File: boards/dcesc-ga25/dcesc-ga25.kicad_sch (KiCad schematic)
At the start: 11 parts, among them J1 Conn_01x03, J2 Conn_01x03, U1 CH32V003J4M6

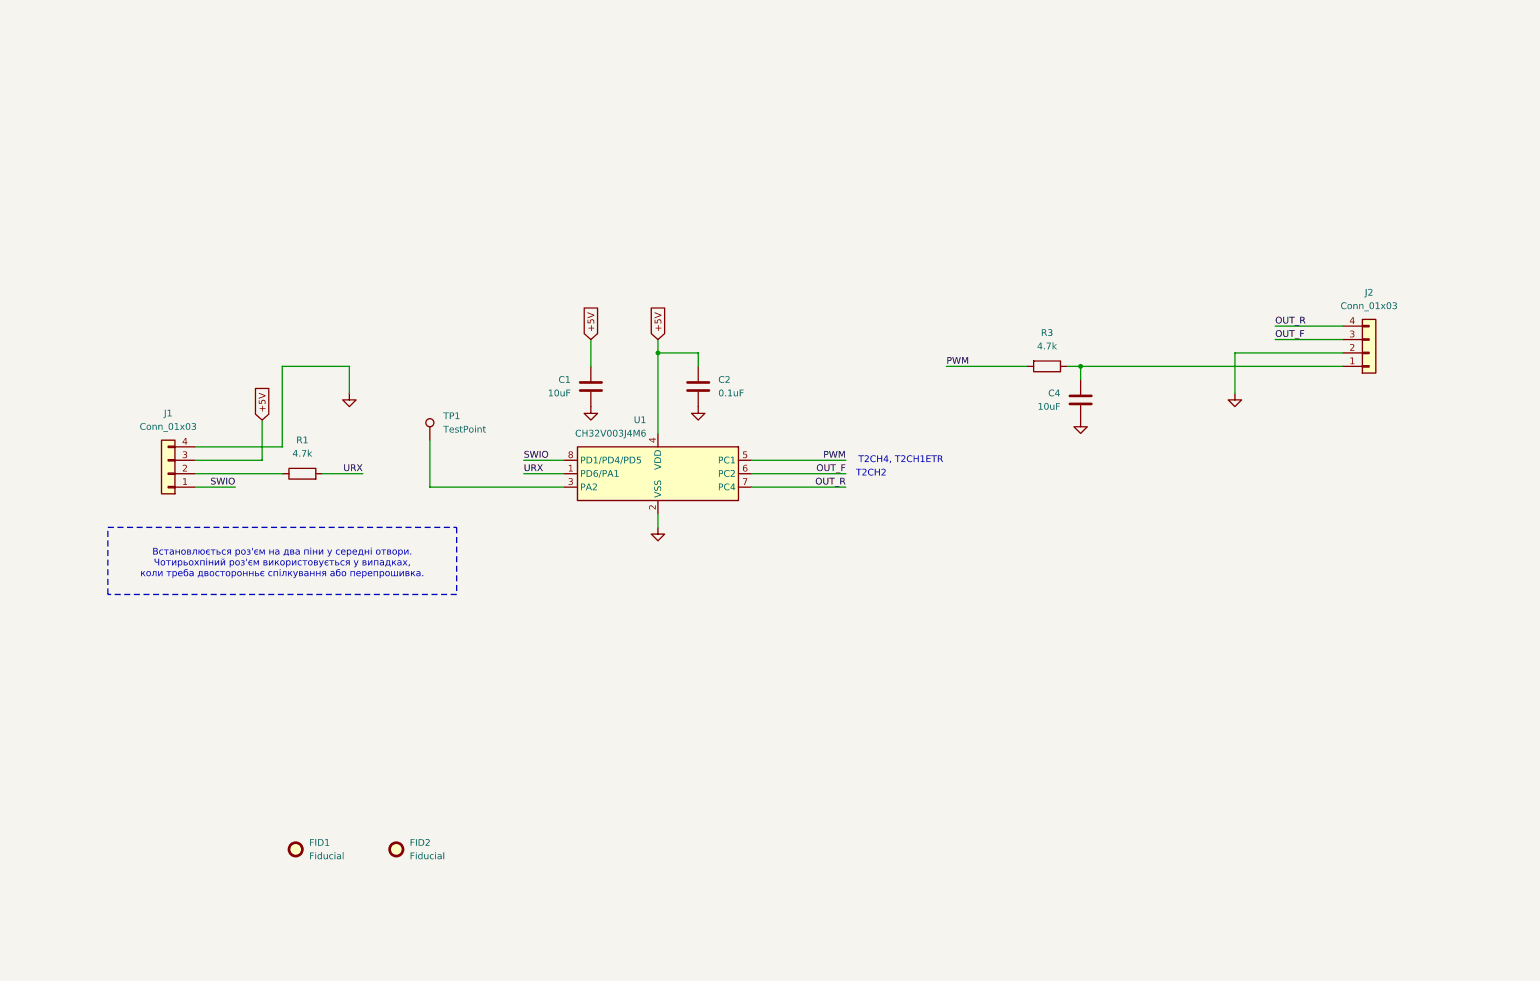
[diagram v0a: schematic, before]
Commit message: Розведено.
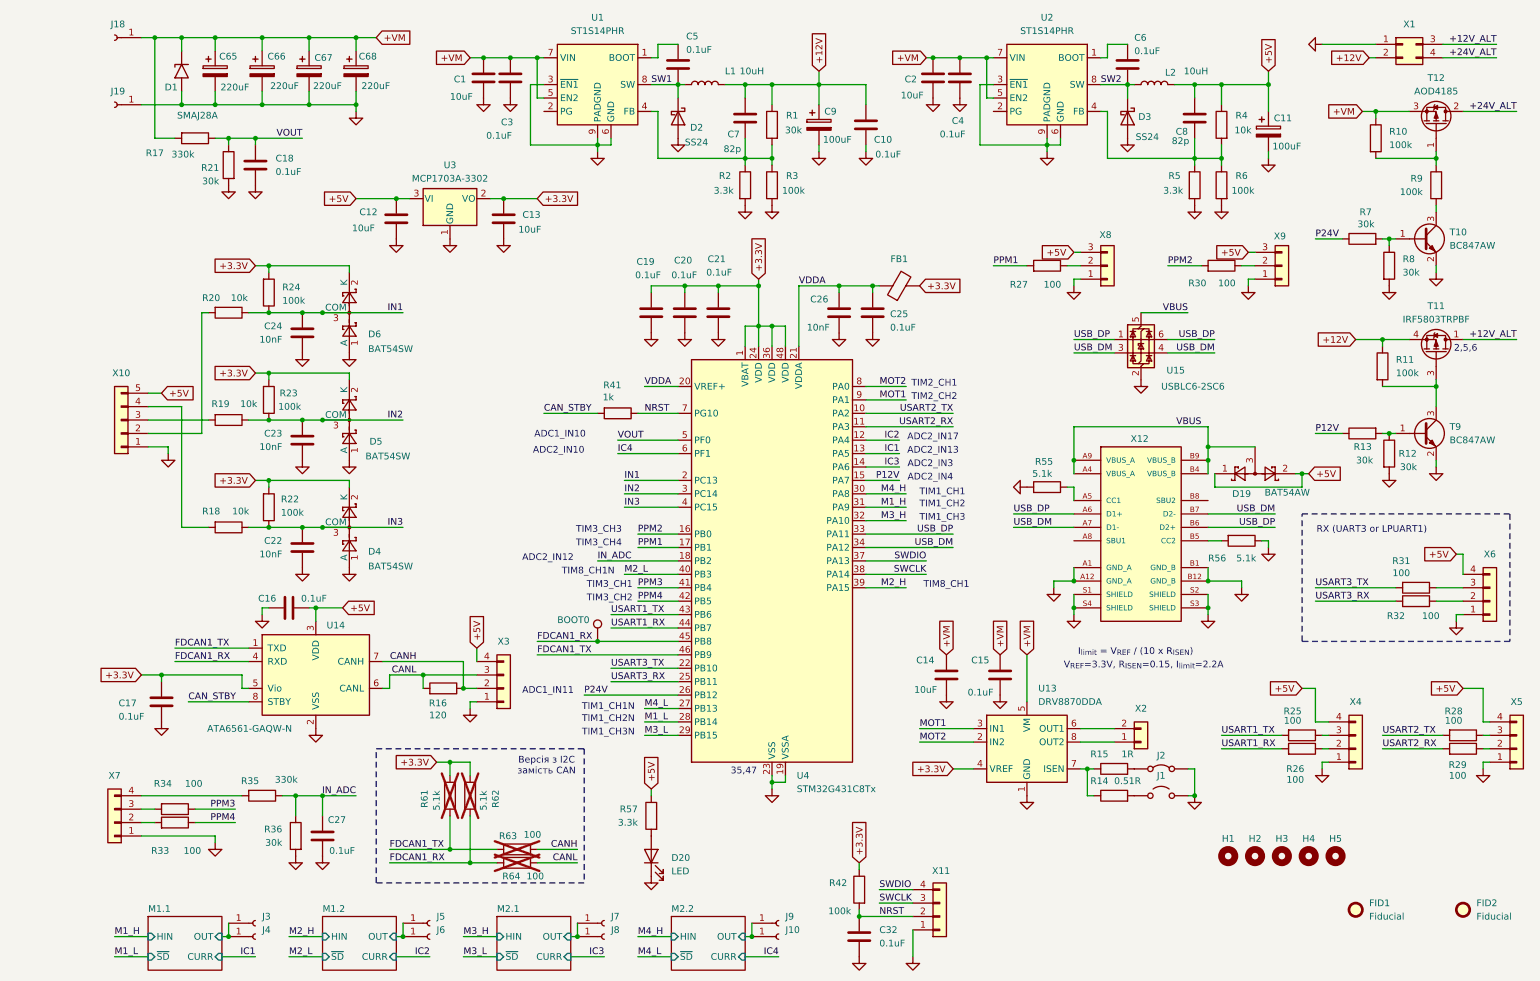
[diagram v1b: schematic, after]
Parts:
- removed J2: Conn_01x03, Connector_JST:JST_PH_S4B-PH-K_1x04_P2.00mm_Horizontal, symbol Connector_Generic:Conn_01x04
- removed U1: CH32V003J4M6, Package_SO:SOP-8_3.9x4.9mm_P1.27mm, symbol MCU_WCH_CH32V0:CH32V003JxMx
- added C1, C14: 10uF, Capacitor_SMD:C_1206_3216Metric, symbol Device:C
- added C10, C15, C16, C17, C18, C19, C20, C21, C25, C27, C3, C32, C5, C6: 0.1uF, Capacitor_SMD:C_0603_1608Metric, symbol Device:C
- added C11: 100uF, Capacitor_Tantalum_SMD:CP_EIA-3528-12_Kemet-T, symbol Device:C_Polarized
- added C12, C13: 10uF, Capacitor_SMD:C_0805_2012Metric, symbol Device:C
- added C22, C23, C24: 10nF, Capacitor_SMD:C_0603_1608Metric, symbol Device:C
- added C65, C66, C67, C68: 220uF, Capacitor_THT:CP_Radial_D10.0mm_P5.00mm, symbol Device:C_Polarized
- added C7, C8: 82p, Capacitor_SMD:C_0603_1608Metric, symbol Device:C
- added C9: 100uF, Capacitor_Tantalum_SMD:CP_EIA-7343-15_Kemet-W, symbol Device:C_Polarized
- added D1: SMAJ28A, Diode_SMD:D_SMA, symbol Diode:SMAJ28A
- added D19: BAT54AW, Package_TO_SOT_SMD:SOT-323_SC-70, symbol Diode:BAT54AW
- added D2, D3: SS24, Diode_SMD:D_SMA, symbol Diode:SS24
- added D20: LED, LED_SMD:LED_0805_2012Metric, symbol Device:LED
- added D4, D5, D6: BAT54SW, Package_TO_SOT_SMD:SOT-323_SC-70, symbol Diode:BAT54SW
- added FB1: FerriteBead, Inductor_SMD:L_0603_1608Metric, symbol Device:FerriteBead
- added H1, H2, H3, H4, H5: MountingHole, MountingHole:MountingHole_3.2mm_M3, symbol Mechanical:MountingHole
- added J1: Jumper_2_Open, Jumper:SolderJumper-2_P1.3mm_Open_RoundedPad1.0x1.5mm, symbol Jumper:Jumper_2_Open
- added J10, J3, J4, J5, J6, J7, J8, J9: Conn_01x01_Socket, Connector_Wire:SolderWire-2.5sqmm_1x01_D2.4mm_OD4.4mm, symbol Connector:Conn_01x01_Socket
- added J18, J19: Conn_01x01_Socket, Connector_Wire:SolderWire-6sqmm_1x01_D3.5mm_OD7mm, symbol Connector:Conn_01x01_Socket
- added J2: Jumper_2_Bridged, Jumper:SolderJumper-2_P1.3mm_Bridged_RoundedPad1.0x1.5mm, symbol Jumper:Jumper_2_Bridged
- added L1, L2: 10uH, locals:Inductor_NR6028T100M, symbol Device:L
- added R10, R11, R22, R23, R24, R42, R6, R9: 100k, Resistor_SMD:R_0603_1608Metric, symbol Device:R
- added R12, R13, R21, R36, R7, R8: 30k, Resistor_SMD:R_0603_1608Metric, symbol Device:R
- added R14: 0.51R, Resistor_SMD:R_1206_3216Metric, symbol Device:R
- added R15: 1R, Resistor_SMD:R_1206_3216Metric, symbol Device:R
- added R16: 120, Resistor_SMD:R_0603_1608Metric, symbol Device:R
- added R17, R35: 330k, Resistor_SMD:R_0603_1608Metric, symbol Device:R
- added R18, R19, R20, R4: 10k, Resistor_SMD:R_0603_1608Metric, symbol Device:R
- added R2, R5, R57: 3.3k, Resistor_SMD:R_0603_1608Metric, symbol Device:R
- added R25, R26, R27, R28, R29, R30, R31, R32, R33, R34, R63, R64: 100, Resistor_SMD:R_0603_1608Metric, symbol Device:R
- added R41: 1k, Resistor_SMD:R_0603_1608Metric, symbol Device:R
- added R55, R56, R61, R62: 5.1k, Resistor_SMD:R_0603_1608Metric, symbol Device:R
- added T10, T9: BC847AW, Package_TO_SOT_SMD:SOT-323_SC-70, symbol Transistor_BJT:BC847W
- added T11: IRF5803TRPBF, Package_SO:TSOP-6_1.65x3.05mm_P0.95mm, symbol Transistor_FET:IRFTS9342PBF
- added T12: AOD4185, Package_TO_SOT_SMD:TO-252-2, symbol Transistor_FET:SUD45P03-09
- added U1, U2: ST1S14PHR, Package_SO:TI_SO-PowerPAD-8, symbol Regulator_Switching:ST1S14PHR
- added U13: DRV8870DDA, Package_SO:Texas_HTSOP-8-1EP_3.9x4.9mm_P1.27mm_EP2.95x4.9mm_Mask2.4x3.1mm_ThermalVias, symbol Driver_Motor:DRV8870DDA
- added U14: ATA6561-GAQW-N, Package_SO:SOIC-8_3.9x4.9mm_P1.27mm, symbol Interface_CAN_LIN:MCP2562-E-SN
- added U15: USBLC6-2SC6, Package_TO_SOT_SMD:SOT-23-6, symbol Power_Protection:USBLC6-2SC6
- added U3: MCP1703A-3302, locals:MCP1703, symbol LocalBaden:MCP1703A-3302_SOT23-regul_0
- added U4: STM32G431C8Tx, Package_QFP:LQFP-48_7x7mm_P0.5mm, symbol MCU_ST_STM32G4:STM32G431C8Tx
- added X1: Conn_02x02_Top_Bottom, Connector_Molex:Molex_Micro-Fit_3.0_43045-0412_2x02_P3.00mm_Vertical, symbol Connector_Generic:Conn_02x02_Top_Bottom
- added X11, X3, X4, X5, X6, X7: Conn_01x03, Connector_JST:JST_ZH_B4B-ZR_1x04_P1.50mm_Vertical, symbol Connector_Generic:Conn_01x04
- added X12: USB4120-03-C_REVA, locals:GCT_USB4120-03-C_REVA, symbol USB4120-03-C_REVA:USB4120-03-C_REVA
- added X2: Conn_01x03, Connector_JST:JST_XH_B2B-XH-AM_1x02_P2.50mm_Vertical, symbol Connector_Generic:Conn_01x02
- added X8, X9: Conn_01x03, Connector_JST:JST_ZH_B3B-ZR_1x03_P1.50mm_Vertical, symbol Connector_Generic:Conn_01x03
- C2: value 0.1uF -> 10uF; footprint Capacitor_SMD:C_0603_1608Metric -> Capacitor_SMD:C_1206_3216Metric
- C26: renamed from C1; value 10uF -> 10nF; footprint Capacitor_SMD:C_0805_2012Metric -> Capacitor_SMD:C_0603_1608Metric
- C4: value 10uF -> 0.1uF; footprint Capacitor_SMD:C_0805_2012Metric -> Capacitor_SMD:C_0603_1608Metric
- R1: value 4.7k -> 30k
- R3: value 4.7k -> 100k
- TP1: value TestPoint -> BOOT0; footprint TestPoint:TestPoint_Pad_2.0x2.0mm -> TestPoint:TestPoint_Pad_1.0x1.0mm
- X10: renamed from J1; footprint Connector_JST:JST_PH_S4B-PH-K_1x04_P2.00mm_Horizontal -> Connector_JST:JST_ZH_B5B-ZR_1x05_P1.50mm_Vertical; symbol Connector_Generic:Conn_01x04 -> Connector_Generic:Conn_01x05
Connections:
- net PWM is gone; now on net GND: R3.2
- net SWIO is gone; now on net GND: X10.1 (Pin_1)
- net URX is gone; now on an unnamed net: R1.2
- net +5V: now also X10.5 (Pin_5), C11.1, C12.1, C16.1, C8.1, D19.1, D19.2, L2.2, R4.1, R57.1, U14.3 (VDD), U3.3 (VI), X3.4 (Pin_4), X4.4 (Pin_4), X5.4 (Pin_4), X6.4 (Pin_4), X8.3 (Pin_3), X9.3 (Pin_3); no longer C2.1, C26.1, X10.3 (Pin_3)
- net GND: now also C1.2, C10.2, C11.2, C12.2, C13.2, C14.2, C15.2, C16.2, C17.2, C18.2, C19.2, C20.2, C21.2, C22.2, C23.2, C24.2, C25.2, C27.2, C3.2, C32.2, C65.2, C66.2, C67.2, C68.2, C9.2, D1.2 (A2), D2.2 (A), D20.1 (K), D3.2 (A), D4.1 (A), D5.1 (A), D6.1 (A), J1.2 (B), J19.1 (Pin_1), J2.2 (B), R12.2, R2.2, R21.2, R36.2, R5.2, R55.2, R56.1, R6.2, R8.2, T10.2 (E), T9.2 (E), U1.3 (~{EN1}), U1.6 (GND), U1.9 (PADGND), U13.1 (GND), U13.9 (GND), U14.2 (VSS), U15.2 (GND), U2.3 (~{EN1}), U2.6 (GND), U2.9 (PADGND), U3.1 (GND), U4.19 (VSSA), U4.23 (VSS), U4.35 (VSS), U4.47 (VSS), X1.1 (Pin_1), X11.1 (Pin_1), X12.A1 (GND_A), X12.A12 (GND_A), X12.B1 (GND_B), X12.B12 (GND_B), X12.S1 (SHIELD), X12.S2 (SHIELD), X12.S3 (SHIELD), X12.S4 (SHIELD), X3.1 (Pin_1), X4.1 (Pin_1), X5.1 (Pin_1), X6.1 (Pin_1), X7.1 (Pin_1), X8.1 (Pin_1), X9.1 (Pin_1); no longer X10.4 (Pin_4)
- net at X10.2 (Pin_2): now also R20.2; no longer R1.1
- net FDCAN1_RX: now reaches TP1.1
- net FDCAN1_RX: now also R62.2, R64.2, U14.4 (RXD), U4.45 (PB8)
- net at R3.1: now also C7.2, R2.1, U1.4 (FB); no longer C4.1
- new net: R55.1, X12.A5 (CC1)
- new net: R56.2, X12.B5 (CC2)
- new net: R32.1, X6.2 (Pin_2)
- new net: R31.1, X6.3 (Pin_3)
- new net: R14.1, R15.1, U13.7 (ISEN)
- new net: J1.1 (A), R14.2
- new net: C8.2, R4.2, R5.1, R6.1, U2.4 (FB)
- new net: R10.2, R9.1, T12.1 (G)
- new net: R9.2, T10.3 (C)
- new net: R27.1, X8.2 (Pin_2)
- new net: R35.2, X7.4 (Pin_4)
- new net: R29.1, X5.2 (Pin_2)
- new net: R28.1, X5.3 (Pin_3)
- new net: R33.2, X7.2 (Pin_2)
- new net: R34.2, X7.3 (Pin_3)
- new net: D20.2 (A), R57.2
- new net: J2.1 (A), R15.2
- new net: C5.1, U1.1 (BOOT)
- new net: R19.2, X10.3 (Pin_3)
- new net: R18.2, X10.4 (Pin_4)
- new net: R25.1, X4.3 (Pin_3)
- new net: C6.1, U2.1 (BOOT)
- new net: R26.1, X4.2 (Pin_2)
- new net: R12.1, R13.2, T9.1 (B)
- new net: U13.8 (OUT2), X2.1 (Pin_1)
- new net: U13.6 (OUT1), X2.2 (Pin_2)
- new net: R11.2, T11.3 (G), T9.3 (C)
- new net: R7.2, R8.1, T10.1 (B)
- new net: R30.1, X9.2 (Pin_2)
- new net +12V: C10.1, C7.1, C9.1, L1.2, R1.1, R11.1, T11.4 (S), X1.2 (Pin_2)
- new net +12V_ALT: T11.1 (D), T11.2 (D), T11.5 (D), T11.6 (D), X1.3 (Pin_3)
- new net +24V_ALT: T12.2 (D), X1.4 (Pin_4)
- new net +3.3V: C13.1, C17.1, C19.1, C20.1, C21.1, D4.2 (K), D5.2 (K), D6.2 (K), FB1.2, R22.2, R23.2, R24.2, R42.1, R61.1, R62.1, U13.4 (VREF), U14.5 (Vio), U3.2 (VO), U4.1 (VBAT), U4.24 (VDD), U4.36 (VDD), U4.48 (VDD)
- new net +VM: C1.1, C14.1, C15.1, C2.1, C3.1, C4.1, C65.1, C66.1, C67.1, C68.1, D1.1 (A1), J18.1 (Pin_1), R10.1, R17.2, T12.3 (S), U1.5 (EN2), U1.7 (VIN), U13.5 (VM), U2.5 (EN2), U2.7 (VIN)
- new net CANH: R16.1, R63.2, U14.7 (CANH), X3.2 (Pin_2)
- new net CANL: R16.2, R64.1, U14.6 (CANL), X3.3 (Pin_3)
- new net CAN_STBY: R41.2, U14.8 (STBY)
- new net FDCAN1_TX: R61.2, R63.1, U14.1 (TXD), U4.46 (PB9)
- new net IC1: U4.13 (PA5)
- new net IC2: U4.12 (PA4)
- new net IC3: U4.14 (PA6)
- new net IC4: U4.6 (PF1)
- new net IN1: C24.1, D6.3 (COM), R20.1, R24.1, U4.2 (PC13)
- new net IN2: C23.1, D5.3 (COM), R19.1, R23.1, U4.3 (PC14)
- new net IN3: C22.1, D4.3 (COM), R18.1, R22.1, U4.4 (PC15)
- new net IN_ADC: C27.1, R35.1, R36.1, U4.18 (PB2)
- new net M1.1/OUT: J3.1 (Pin_1), J4.1 (Pin_1)
- new net M1.2/OUT: J5.1 (Pin_1), J6.1 (Pin_1)
- new net M1_H: U4.31 (PA9)
- new net M1_L: U4.28 (PB14)
- new net M2.1/OUT: J7.1 (Pin_1), J8.1 (Pin_1)
- new net M2.2/OUT: J10.1 (Pin_1), J9.1 (Pin_1)
- new net M2_H: U4.39 (PA15)
- new net M2_L: U4.40 (PB3)
- new net M3_H: U4.32 (PA10)
- new net M3_L: U4.29 (PB15)
- new net M4_H: U4.30 (PA8)
- new net M4_L: U4.27 (PB13)
- new net MOT1: U13.3 (IN1), U4.9 (PA1)
- new net MOT2: U13.2 (IN2), U4.8 (PA0)
- new net NRST: C32.1, R41.1, R42.2, U4.7 (PG10), X11.2 (Pin_2)
- new net P12V: R13.1, U4.15 (PA7)
- new net P24V: R7.1, U4.26 (PB12)
- new net PPM1: R27.2, U4.17 (PB1)
- new net PPM2: R30.2, U4.16 (PB0)
- new net PPM3: R34.1, U4.41 (PB4)
- new net PPM4: R33.1, U4.42 (PB5)
- new net SW1: C5.2, D2.1 (K), L1.1, U1.8 (SW)
- new net SW2: C6.2, D3.1 (K), L2.1, U2.8 (SW)
- new net SWCLK: U4.38 (PA14), X11.3 (Pin_3)
- new net SWDIO: U4.37 (PA13), X11.4 (Pin_4)
- new net USART1_RX: R26.2, U4.44 (PB7)
- new net USART1_TX: R25.2, U4.43 (PB6)
- new net USART2_RX: R29.2, U4.11 (PA3)
- new net USART2_TX: R28.2, U4.10 (PA2)
- new net USART3_RX: R32.2, U4.25 (PB11)
- new net USART3_TX: R31.2, U4.22 (PB10)
- new net USB_DM: U15.3 (I/O2), U15.4 (I/O2), U4.34 (PA12), X12.A7 (D1-), X12.B7 (D2-)
- new net USB_DP: U15.1 (I/O1), U15.6 (I/O1), U4.33 (PA11), X12.A6 (D1+), X12.B6 (D2+)
- new net VBUS: D19.3, U15.5 (VBUS), X12.A4 (VBUS_A), X12.A9 (VBUS_A), X12.B4 (VBUS_B), X12.B9 (VBUS_B)
- new net VDDA: C25.1, C26.1, FB1.1, U4.20 (VREF+), U4.21 (VDDA)
- new net VOUT: C18.1, R17.1, R21.1, U4.5 (PF0)
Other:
- added sheet M1.1 (m-channel.kicad_sch)
- added sheet M1.2 (m-channel.kicad_sch)
- added sheet M2.1 (m-channel.kicad_sch)
- added sheet M2.2 (m-channel.kicad_sch)
- note added: "2,5,6"
- note added: "35,47"
- note added: "ADC1_IN10"
- note added: "ADC1_IN11"
- note added: "ADC2_IN10"
- note added: "ADC2_IN12"
- note added: "ADC2_IN13"
- note added: "ADC2_IN17"
- note added: "ADC2_IN3"
- note added: "ADC2_IN4"
- note added: "I_{limit} = V_{REF} / (10 x R_{ISEN})"
- note added: "RX (UART3 or LPUART1)"
- note added: "TIM1_CH1"
- note added: "TIM1_CH1N"
- note added: "TIM1_CH2"
- note added: "TIM1_CH2N"
- note added: "TIM1_CH3"
- note added: "TIM1_CH3N"
- note added: "TIM2_CH1"
- note added: "TIM2_CH2"
- note added: "TIM3_CH1"
- note added: "TIM3_CH2"
- note added: "TIM3_CH3"
- note added: "TIM3_CH4"
- note added: "TIM8_CH1"
- note added: "TIM8_CH1N"
- note added: "V_{REF}=3.3V, R_{ISEN}=0.15, I_{limit}=2.2A"
- note added: "Версія з I2C замість CAN"
- note removed: "T2CH2"
- note removed: "T2CH4, T2CH1ETR"
- note removed: "Встановлюється роз'єм на два піни у середні отвори. Чотирьохпіний роз'єм використовується у випадках, коли треба двосторонньє спілкування або перепрошивка."
- moved on the sheet: C26, FID1, FID2
